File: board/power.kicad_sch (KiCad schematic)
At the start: 47 parts, among them U1 AMS1117-3.3, U4 TPS53318DQPR, U5 CH224K

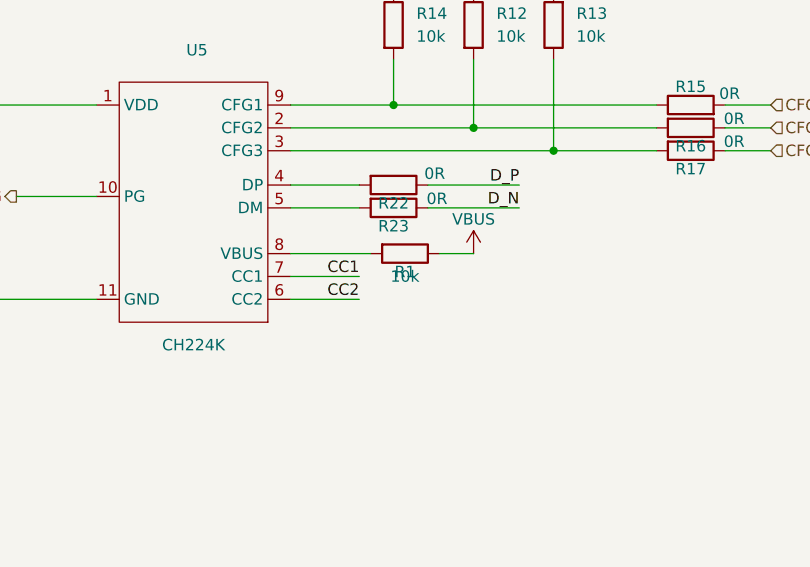
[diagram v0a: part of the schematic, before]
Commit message: Ordered!
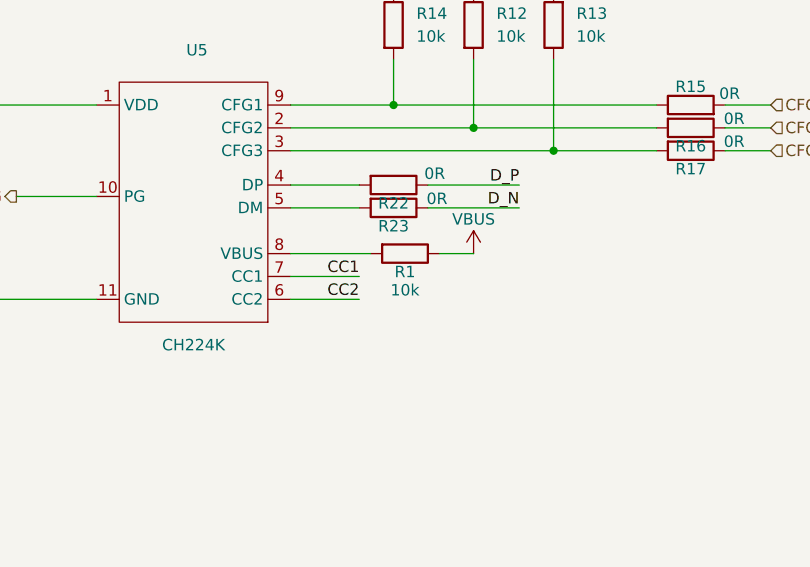
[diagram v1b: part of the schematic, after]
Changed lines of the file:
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@@
 		)
 		(property "Value" "10k"
-			(at 214.63 74.93 90)
+			(at 214.63 76.454 90)
 			(effects
 				(font
